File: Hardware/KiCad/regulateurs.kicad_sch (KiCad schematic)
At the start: 22 parts, among them IC2 MP1475DJ-LF-P, J1 Conn_Battery_Cell

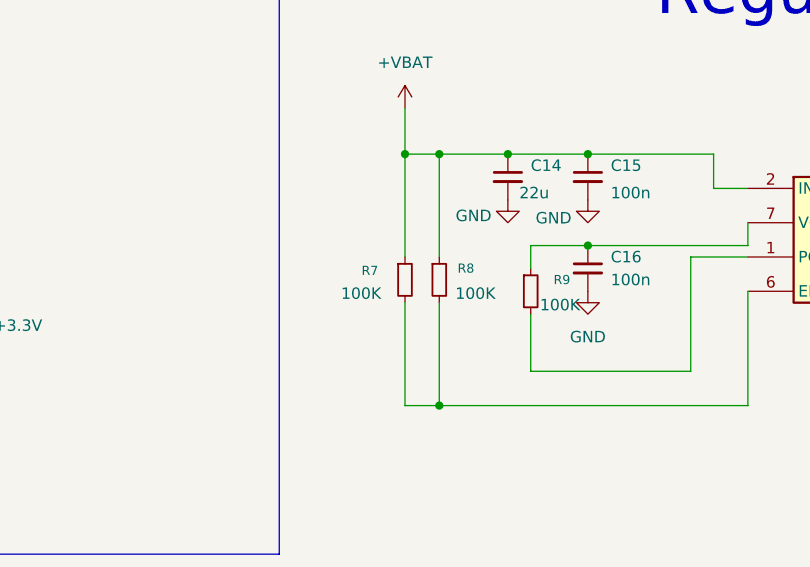
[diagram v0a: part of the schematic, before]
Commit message: sss
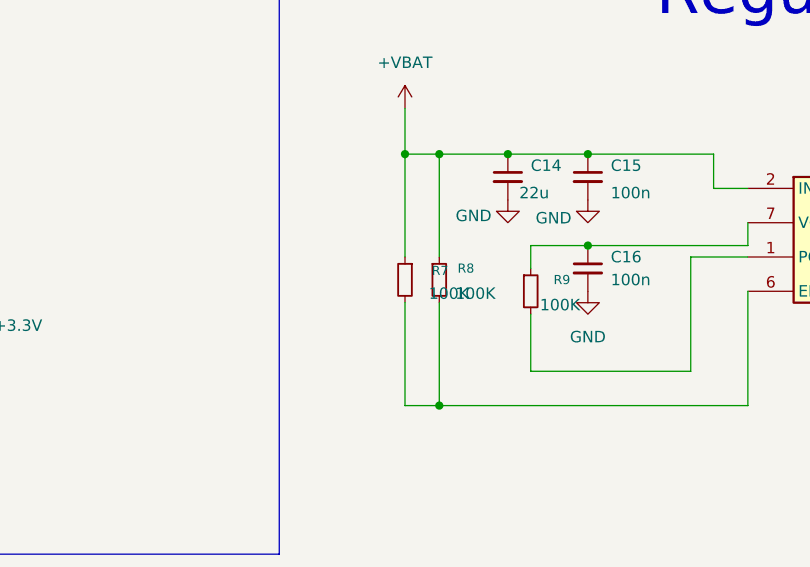
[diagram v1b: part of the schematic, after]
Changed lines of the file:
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@@
 		(lib_id "Device:R_Small")
 		(at 149.86 62.23 0)
+		(mirror y)
 		(unit 1)
 		(exclude_from_sim no)
@@
 		(dnp no)
 		(property "Reference" "R7"
-			(at 145.034 61.214 0)
+			(at 154.686 61.214 0)
 			(effects
 				(font
@@
 		)
 		(property "Value" "100K"
-			(at 142.748 63.754 0)
+			(at 156.972 63.754 0)
 			(effects
 				(font

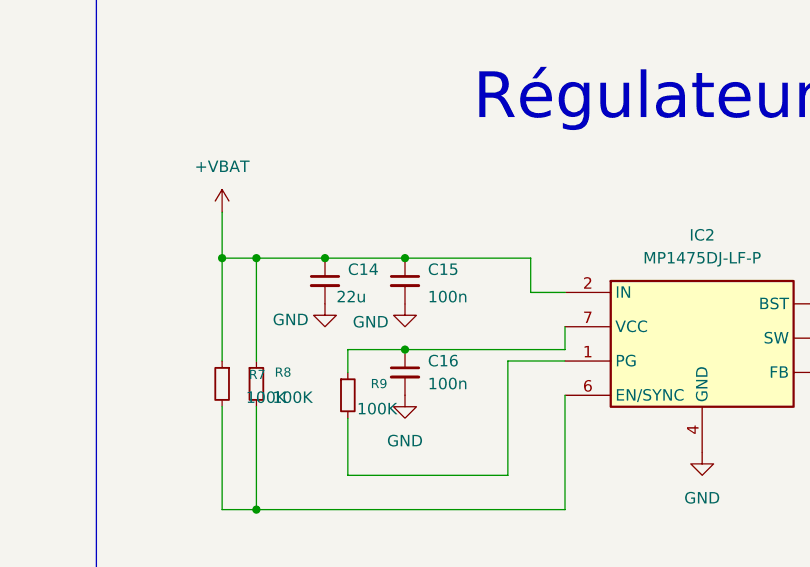
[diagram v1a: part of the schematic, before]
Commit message: R
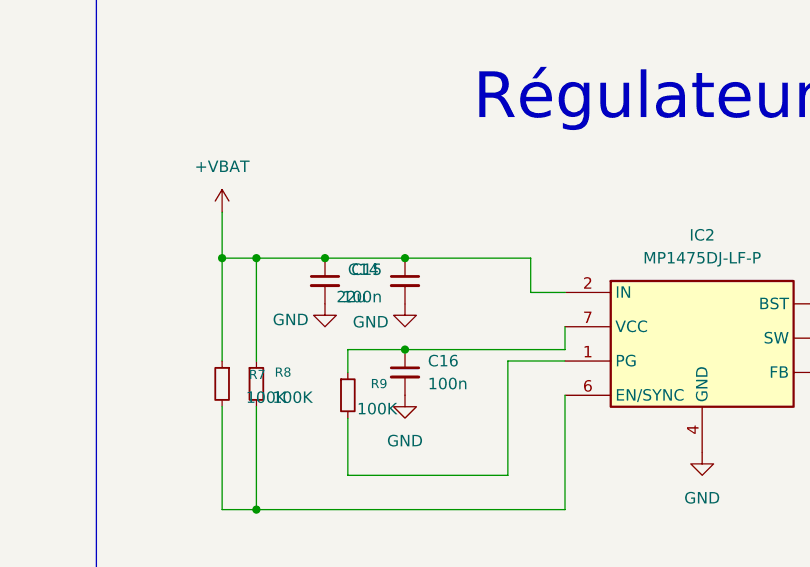
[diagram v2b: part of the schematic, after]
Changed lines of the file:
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@@
 		(lib_id "Device:C_Small")
 		(at 170.18 50.8 0)
+		(mirror y)
 		(unit 1)
 		(exclude_from_sim no)
@@
 		(dnp no)
 		(property "Reference" "C15"
-			(at 172.72 49.5362 0)
+			(at 167.64 49.5362 0)
 			(effects
 				(font
@@
 		)
 		(property "Value" "100n"
-			(at 172.72 52.578 0)
+			(at 167.64 52.578 0)
 			(effects
 				(font
